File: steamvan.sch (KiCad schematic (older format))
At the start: 24 parts, among them J1 Conn_01x05_Male, Q1 FMMT493TA, SW1 SW_Push, U1 STM32F303CBTx, U2 TLV70233_SOT23-5, U3 NUF2221W1T2G, Y1 8MHz

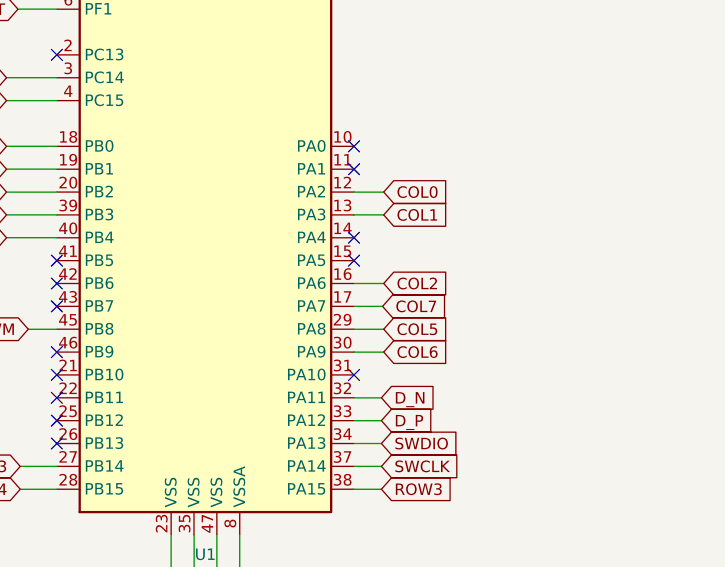
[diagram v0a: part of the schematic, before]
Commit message: Update: Work on routing
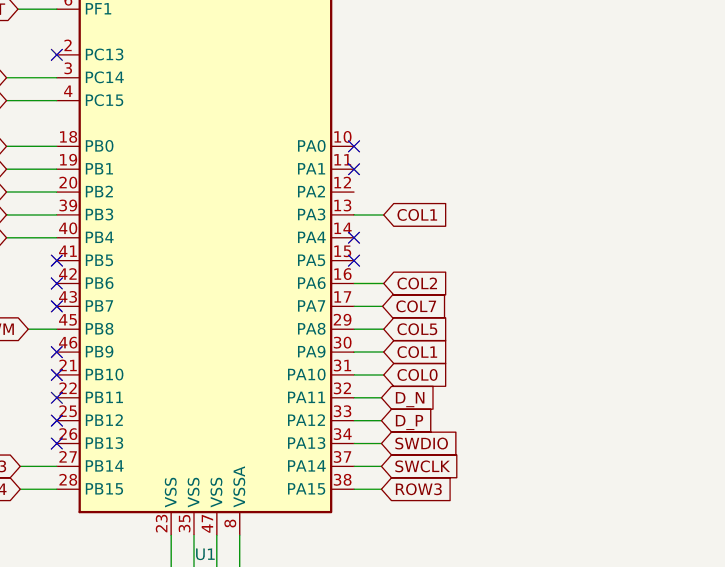
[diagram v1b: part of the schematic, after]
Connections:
- net COL6 is gone; now on net COL1: U1.30 (PA9)
- net COL0: now also U1.31 (PA10); no longer U1.12 (PA2)
- no-connect marks 16 -> 15
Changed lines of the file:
@@
 Wire Wire Line
 	9125 4840 9005 4840
-Text GLabel 9135 3540 2    50   Input ~ 0
+Text GLabel 9135 4340 2    50   Input ~ 0
 COL0
-Wire Wire Line
-	9135 3540 9005 3540
 Text GLabel 9135 3640 2    50   Input ~ 0
 COL1
@@
 COL5
 Text GLabel 9135 4240 2    50   Input ~ 0
-COL6
+COL1
 Wire Wire Line
 	9005 4140 9135 4140
@@
 NoConn ~ 9005 3740
 NoConn ~ 9005 3840
-NoConn ~ 9005 4340
 NoConn ~ 7705 4640
 NoConn ~ 7705 4540
@@
 Wire Wire Line
 	2215 2865 2215 2825
+Wire Wire Line
+	9005 4340 9135 4340
 $EndSCHEMATC

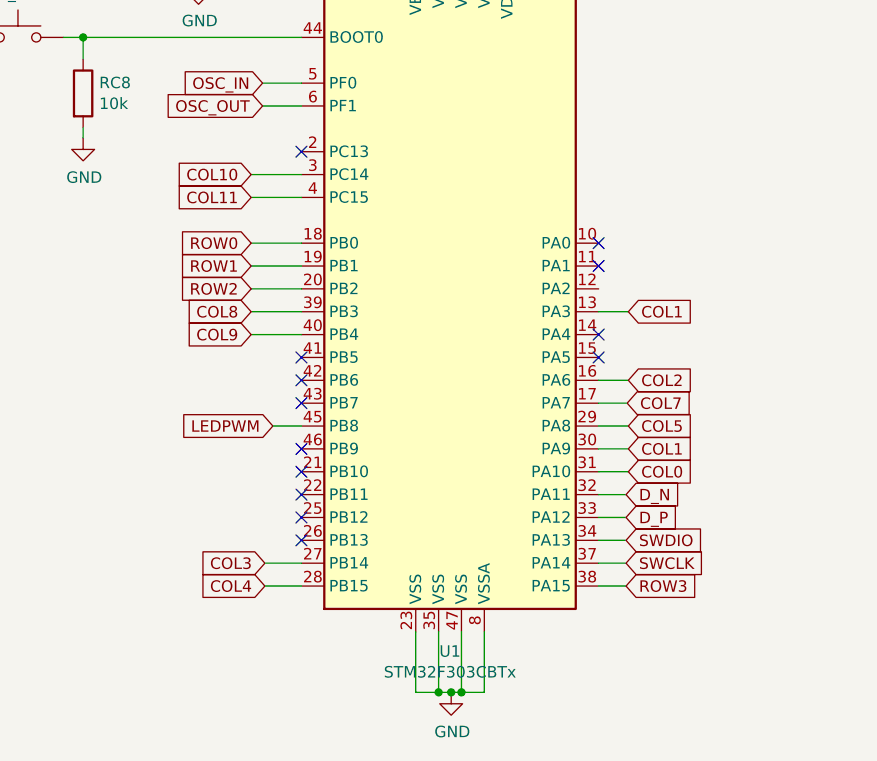
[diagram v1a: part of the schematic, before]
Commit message: Update: Work on routing
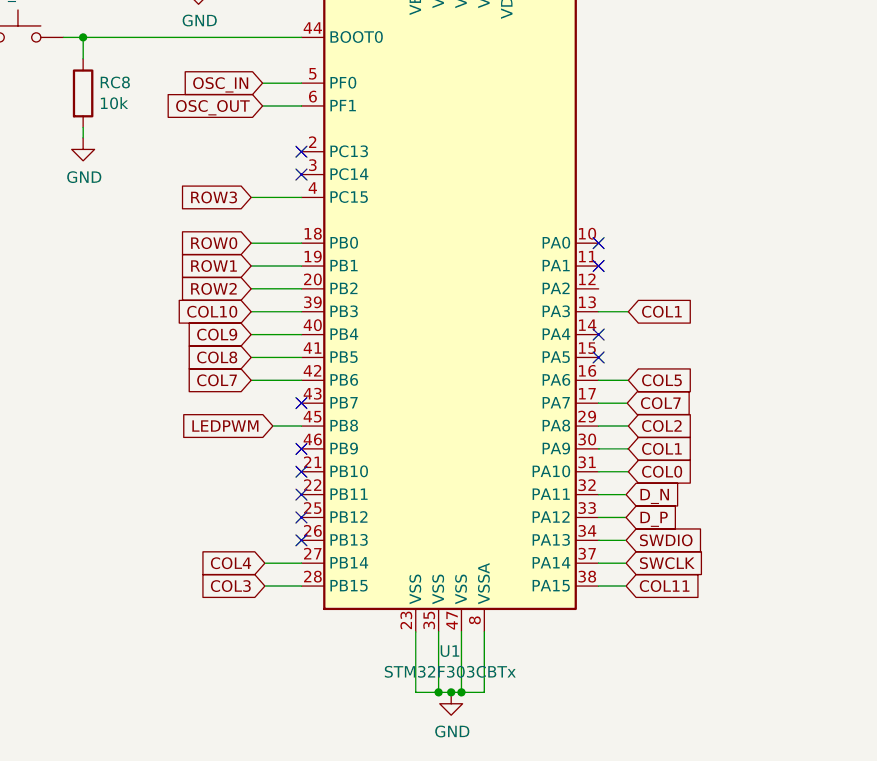
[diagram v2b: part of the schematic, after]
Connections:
- net COL10: now also U1.39 (PB3); no longer U1.3 (PC14)
- net COL11: now also U1.38 (PA15); no longer U1.4 (PC15)
- net COL2: now also U1.29 (PA8); no longer U1.16 (PA6)
- net COL3: now also U1.28 (PB15); no longer U1.27 (PB14)
- net COL4: now also U1.27 (PB14); no longer U1.28 (PB15)
- net COL5: now also U1.16 (PA6); no longer U1.29 (PA8)
- net COL7: now also U1.42 (PB6)
- net COL8: now also U1.41 (PB5); no longer U1.39 (PB3)
- net ROW3: now also U1.4 (PC15); no longer U1.38 (PA15)
- no-connect marks 15 -> 14
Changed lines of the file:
@@
 	7485 3540 7705 3540
 Text GLabel 9125 4840 2    50   Input ~ 0
-ROW3
+COL11
 Wire Wire Line
 	9125 4840 9005 4840
@@
 	9135 3640 9005 3640
 Text GLabel 9135 3940 2    50   Input ~ 0
-COL2
+COL5
 Wire Wire Line
 	9005 3940 9135 3940
 Text GLabel 7545 4740 0    50   Input ~ 0
+COL4
+Text GLabel 7545 4840 0    50   Input ~ 0
 COL3
-Text GLabel 7545 4840 0    50   Input ~ 0
-COL4
 Wire Wire Line
 	7545 4840 7705 4840
@@
 	7545 4740 7705 4740
 Text GLabel 9135 4140 2    50   Input ~ 0
-COL5
+COL2
 Text GLabel 9135 4240 2    50   Input ~ 0
 COL1
@@
 	9005 4040 9130 4040
 Text GLabel 7485 3640 0    50   Input ~ 0
-COL8
-Text GLabel 7485 3740 0    50   Input ~ 0
-COL9
+COL10
 Wire Wire Line
 	7485 3640 7705 3640
-Wire Wire Line
-	7485 3740 7705 3740
-Text GLabel 7485 3040 0    50   Input ~ 0
-COL10
 Text GLabel 7485 3140 0    50   Input ~ 0
-COL11
-Wire Wire Line
-	7485 3040 7705 3040
+ROW3
 Wire Wire Line
 	7485 3140 7705 3140
@@
 NoConn ~ 7705 4240
 NoConn ~ 7705 4040
-NoConn ~ 7705 3940
-NoConn ~ 7705 3840
 $Comp
 L power:PWR_FLAG #FLG0101
@@
 Wire Wire Line
 	9005 4340 9135 4340
+Text GLabel 7485 3840 0    50   Input ~ 0
+COL8
+Wire Wire Line
+	7485 3840 7705 3840
+NoConn ~ 7705 3040
+Text GLabel 7485 3940 0    50   Input ~ 0
+COL7
+Wire Wire Line
+	7485 3740 7705 3740
+Text GLabel 7485 3740 0    50   Input ~ 0
+COL9
+Wire Wire Line
+	7485 3940 7705 3940
 $EndSCHEMATC
